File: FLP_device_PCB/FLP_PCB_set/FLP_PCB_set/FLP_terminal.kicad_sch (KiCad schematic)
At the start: 0 parts

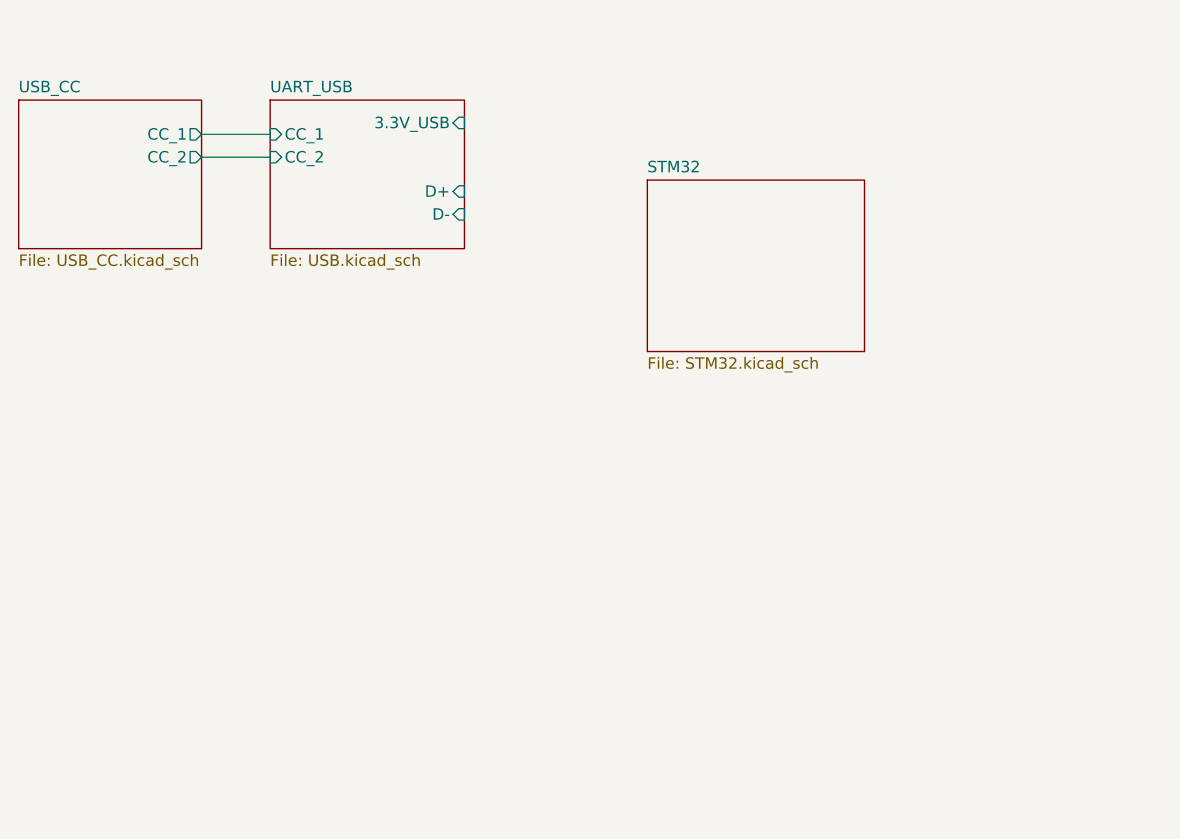
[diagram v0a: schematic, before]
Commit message: FLP_set add
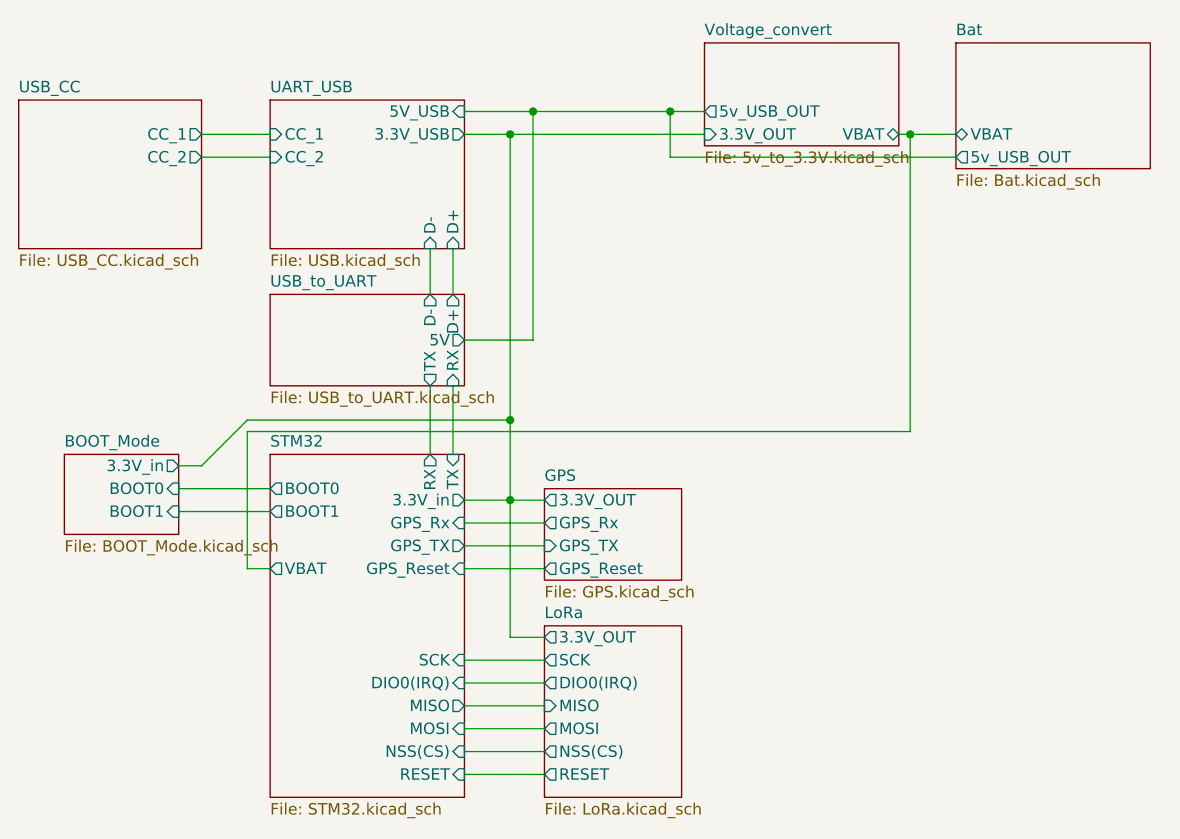
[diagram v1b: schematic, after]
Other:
- added sheet BOOT_Mode (BOOT_Mode.kicad_sch)
- added sheet Bat (Bat.kicad_sch)
- added sheet GPS (GPS.kicad_sch)
- added sheet LoRa (LoRa.kicad_sch)
- added sheet USB_to_UART (USB_to_UART.kicad_sch)
- added sheet Voltage_convert (5v_to_3.3V.kicad_sch)
- sheet STM32 ports: added 3.3V_in, BOOT0, BOOT1, DIO0(IRQ), GPS_Reset, GPS_Rx, GPS_TX, MISO, MOSI, NSS(CS), RESET, RX, SCK, TX, VBAT; removed none
- sheet UART_USB ports: added 5V_USB; removed none
